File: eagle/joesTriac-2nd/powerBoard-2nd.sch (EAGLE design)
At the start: 6 parts, among them J1 XF2E-0815-1

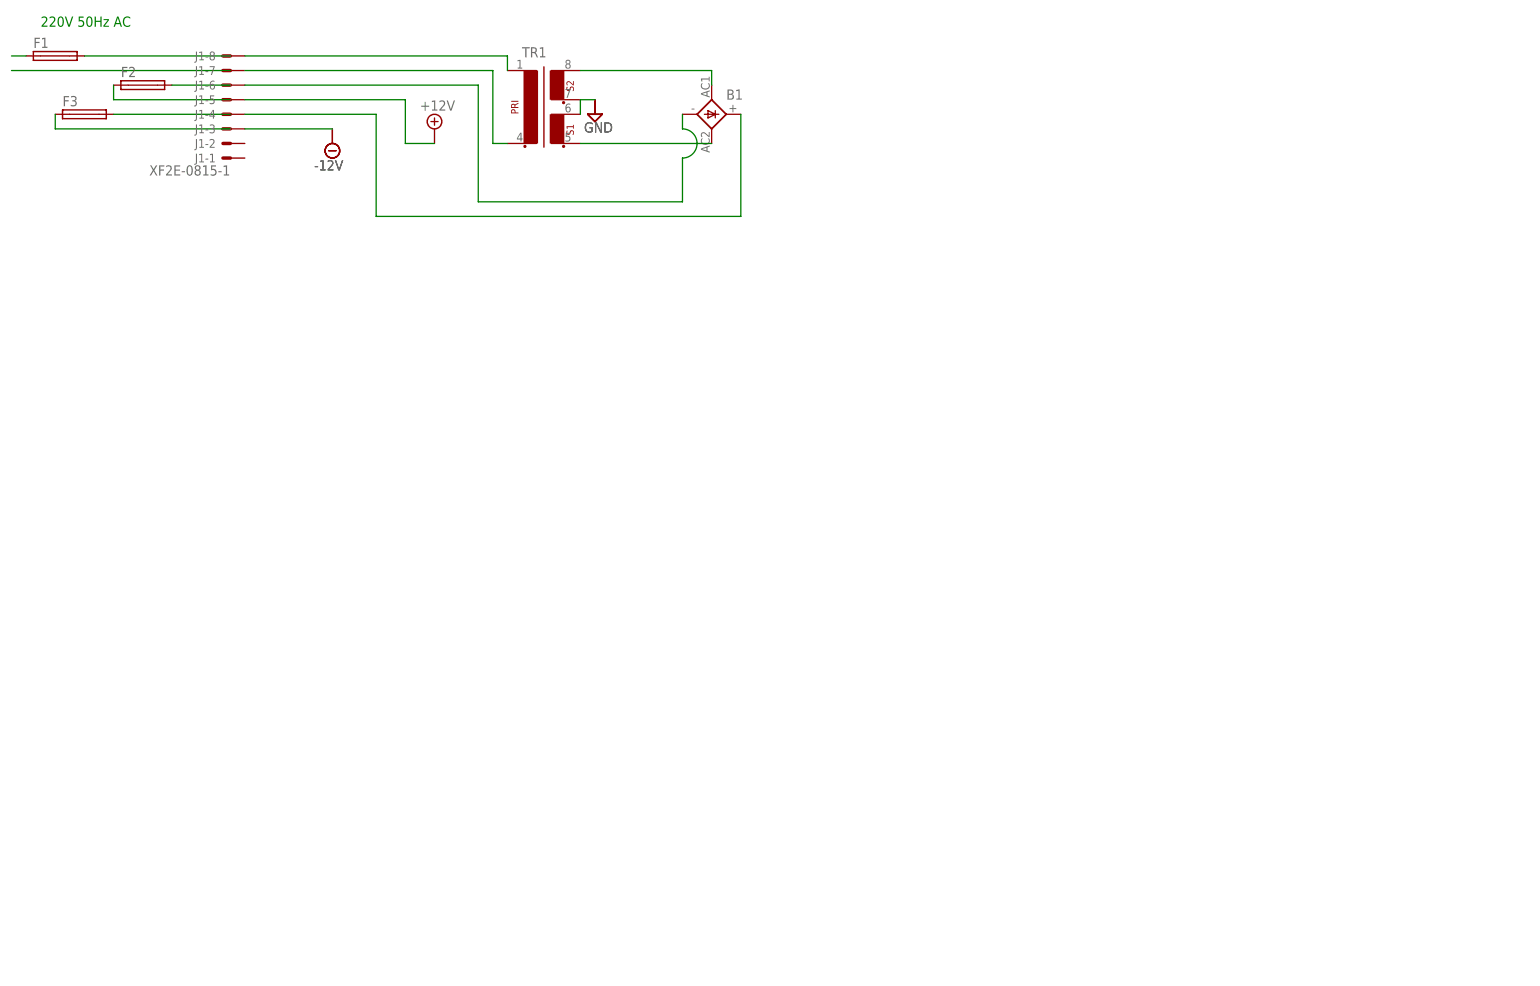
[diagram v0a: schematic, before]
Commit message: reg save
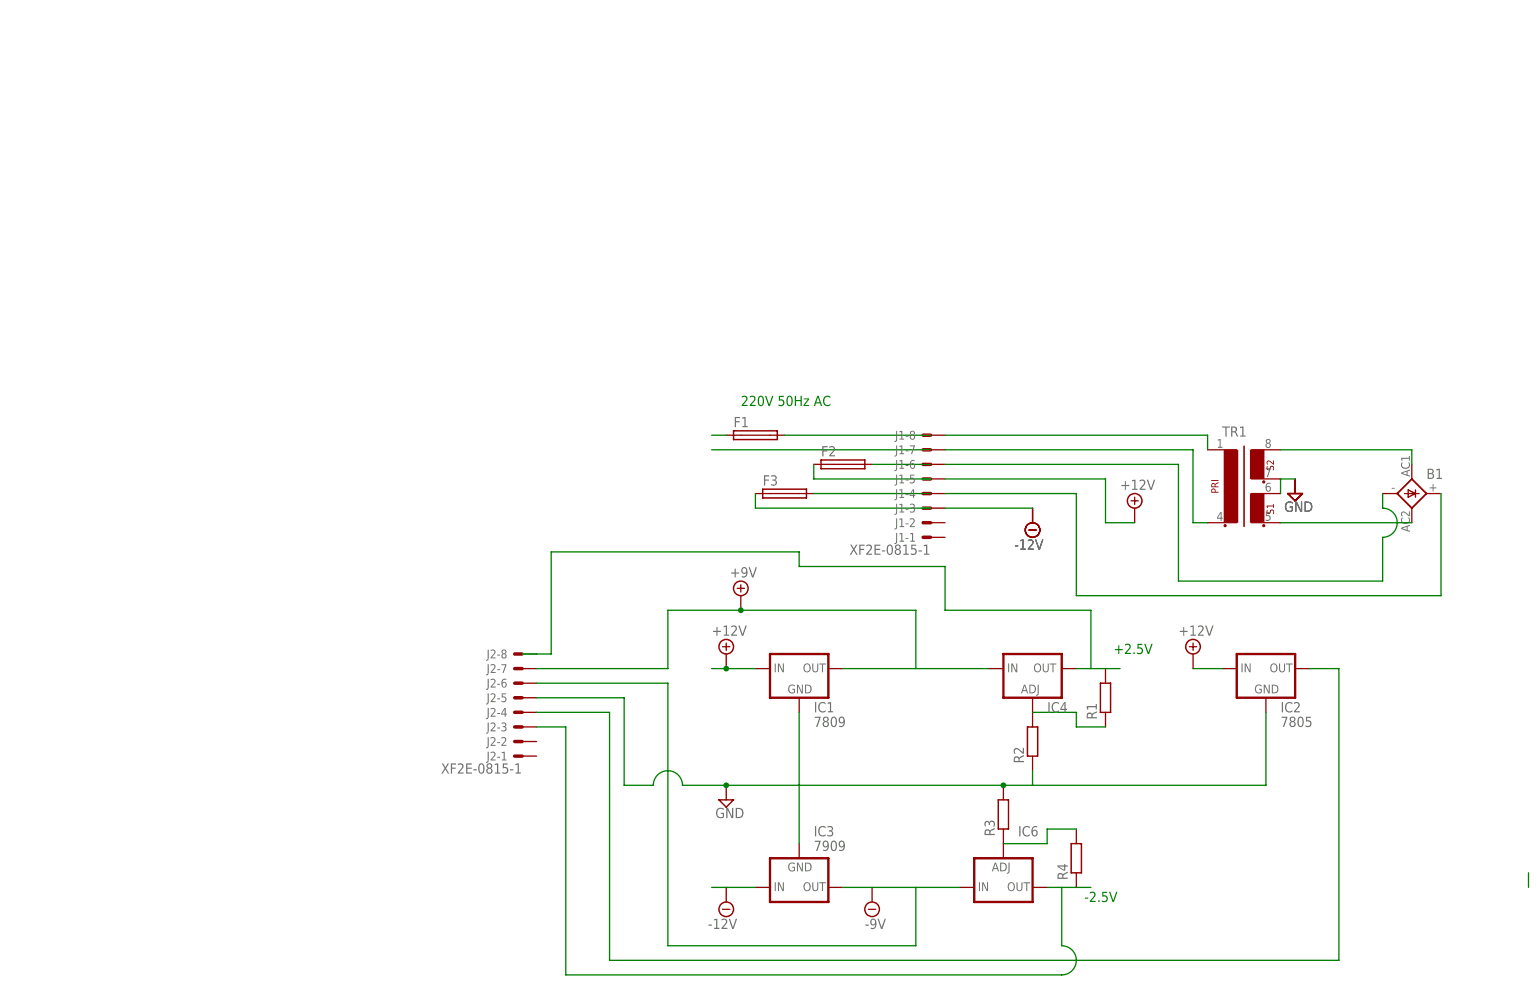
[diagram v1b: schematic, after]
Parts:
- added IC1: 7809, v-reg:78LXX
- added IC2: 7805, v-reg:78LXX
- added IC3: 7909, v-reg:79LXX
- added IC4: (no value), v-reg:LM317-T039
- added IC6: (no value), v-reg:LM337-TO3
- added J2: XF2E-0815-1, con-omron:XF2E-0815-1
- added R1, R2, R3, R4: (no value), resistor:R-EU_0309/V
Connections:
- new net +9V: IC1.OUT, IC4.IN, J2-7.MS
- new net -9V: IC3.OUT, IC6.IN, J2-6.MS
- new net N$10: IC2.OUT, J2-4.MS
- new net N$18: IC4.ADJ, R1.1, R2.2
- new net N$19: IC6.ADJ, R3.1, R4.2
- new net N$21: IC6.OUT, J2-3.MS
- new net N$23: IC4.OUT, J2-8.MS
- net +12V: now also IC1.IN, IC2.IN
- net -12V: now also IC3.IN
- net GND: now also IC1.GND, IC2.GND, IC3.GND, J2-5.MS, R2.1, R3.2
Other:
- note added: "+2.5V"
- note added: "-2.5V"
- moved on the sheet: B1, F1, F2, F3, J1-1, J1-2, J1-3, J1-4, J1-5, J1-6, J1-7, J1-8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
